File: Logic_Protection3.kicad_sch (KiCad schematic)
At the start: 16 parts

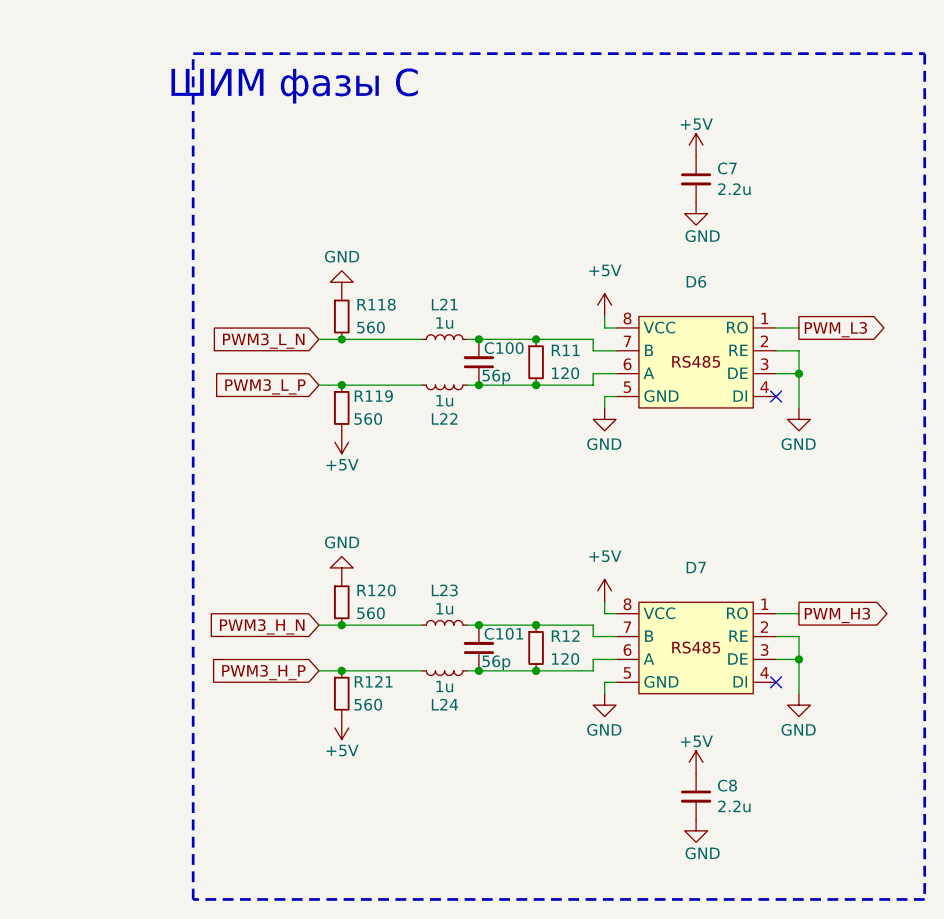
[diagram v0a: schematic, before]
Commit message: VER2.2.1: создал папку для производственных доков
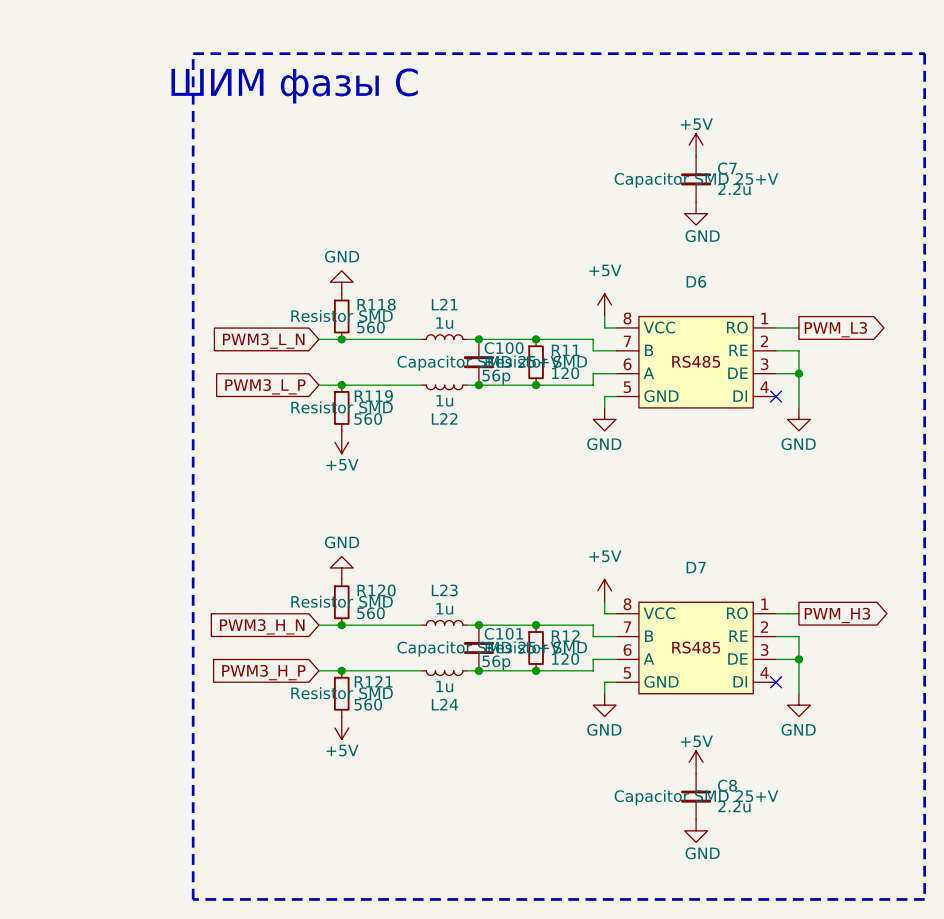
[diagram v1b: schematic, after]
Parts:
- C100, C101, C7, C8: Description P/N (none) -> Capacitor SMD 25+V
- R11, R118, R119, R12, R120, R121: Description P/N (none) -> Resistor SMD
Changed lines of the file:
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@@
 			)
 		)
-		(property "Description P/N" ""
+		(property "Description P/N" "Resistor SMD"
 			(at 132.08 93.98 0)
 			(effects
@@
 			)
 		)
-		(property "Description P/N" ""
+		(property "Description P/N" "Capacitor SMD 25+V"
 			(at 147.32 120.65 0)
 			(effects
@@
 			)
 		)
-		(property "Description P/N" ""
+		(property "Description P/N" "Resistor SMD"
 			(at 153.67 120.65 0)
 			(effects
@@
 			)
 		)
-		(property "Description P/N" ""
+		(property "Description P/N" "Resistor SMD"
 			(at 132.08 125.73 0)
 			(effects
@@
 			)
 		)
-		(property "Description P/N" ""
+		(property "Description P/N" "Resistor SMD"
 			(at 132.08 115.57 0)
 			(effects
@@
 			)
 		)
-		(property "Description P/N" ""
+		(property "Description P/N" "Capacitor SMD 25+V"
 			(at 147.32 88.9 0)
 			(effects
@@
 			)
 		)
-		(property "Description P/N" ""
+		(property "Description P/N" "Capacitor SMD 25+V"
 			(at 171.45 137.16 0)
 			(effects
@@
 			)
 		)
-		(property "Description P/N" ""
+		(property "Description P/N" "Capacitor SMD 25+V"
 			(at 171.45 68.58 0)
 			(effects
@@
 			)
 		)
-		(property "Description P/N" ""
+		(property "Description P/N" "Resistor SMD"
 			(at 132.08 83.82 0)
 			(effects
@@
 			)
 		)
-		(property "Description P/N" ""
+		(property "Description P/N" "Resistor SMD"
 			(at 153.67 88.9 0)
 			(effects

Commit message: VER2.2.1: исправил все доки
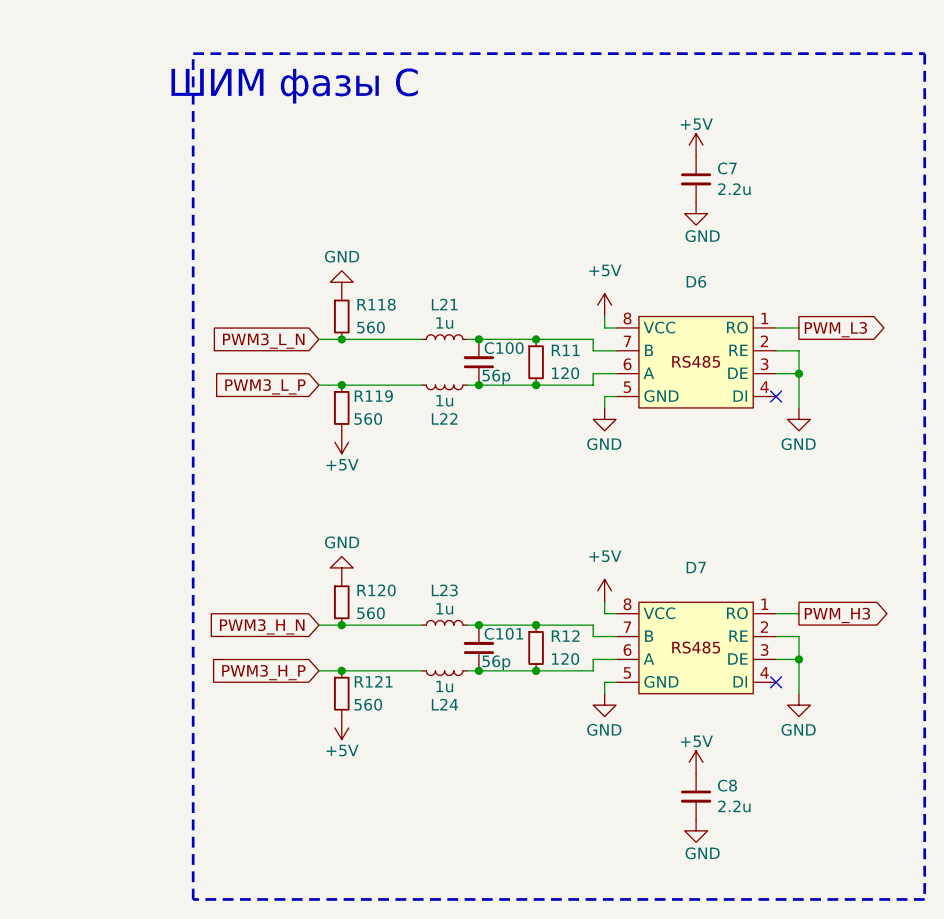
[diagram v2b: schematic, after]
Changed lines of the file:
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@@
 		(date "2025-06-04")
 		(company "ООО \"ЭТТ\"")
+		(comment 1 "НВЦТ.EVP150-2-1.2000.120_v1 Э3")
 	)
 	(rectangle
@@
 					(size 1.27 1.27)
 				)
+				(hide yes)
 			)
 		)
@@
 					(size 1.27 1.27)
 				)
+				(hide yes)
 			)
 		)
@@
 					(size 1.27 1.27)
 				)
+				(hide yes)
 			)
 		)
@@
 					(size 1.27 1.27)
 				)
+				(hide yes)
 			)
 		)
@@
 					(size 1.27 1.27)
 				)
+				(hide yes)
 			)
 		)
@@
 					(size 1.27 1.27)
 				)
+				(hide yes)
 			)
 		)
@@
 					(size 1.27 1.27)
 				)
+				(hide yes)
 			)
 		)
@@
 					(size 1.27 1.27)
 				)
+				(hide yes)
 			)
 		)
@@
 					(size 1.27 1.27)
 				)
+				(hide yes)
 			)
 		)
@@
 					(size 1.27 1.27)
 				)
-			)
-		)
+				(hide yes)
+			)
+		)

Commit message: VER2.2: исправил ошибки в доках
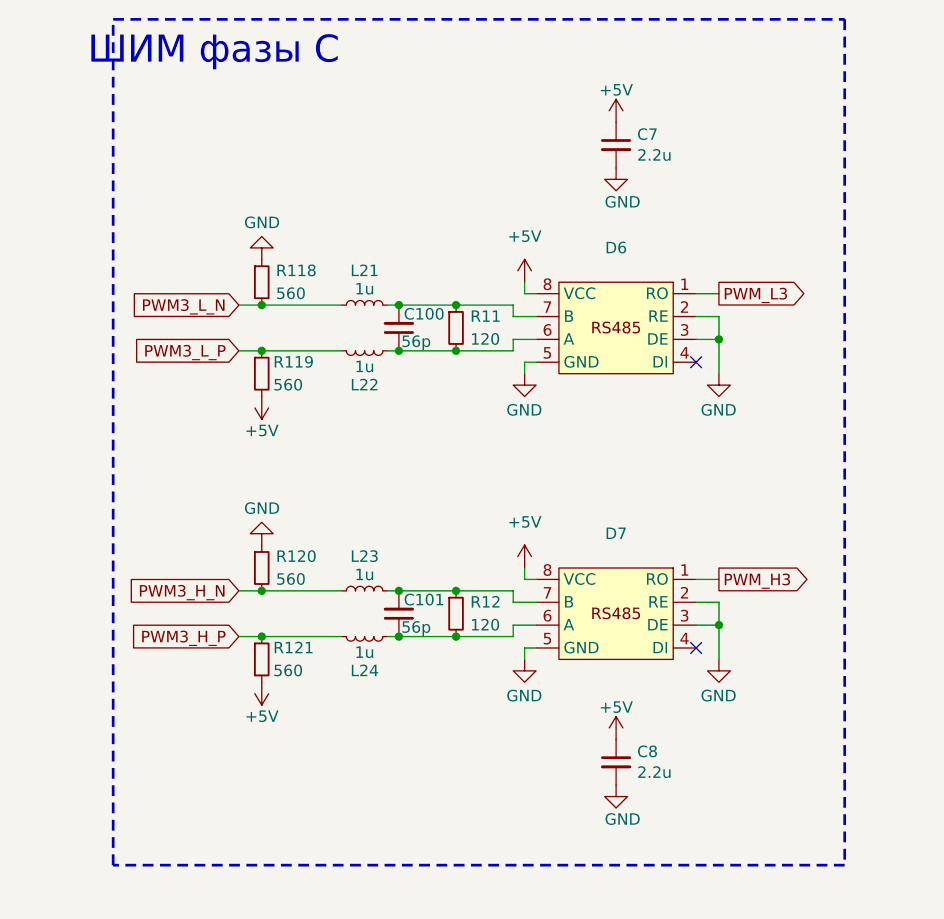
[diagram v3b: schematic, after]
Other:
- moved on the sheet: C100, C101, C7, C8, D6, D7, L21, L22, L23, L24, R11, R118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
